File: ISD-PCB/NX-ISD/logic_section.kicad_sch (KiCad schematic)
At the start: 12 parts, among them J1 1-2328702-0, Q4 AO3400A, U1 ESP32-S3-WROOM-1, U14 ZDSD02GLGEAG

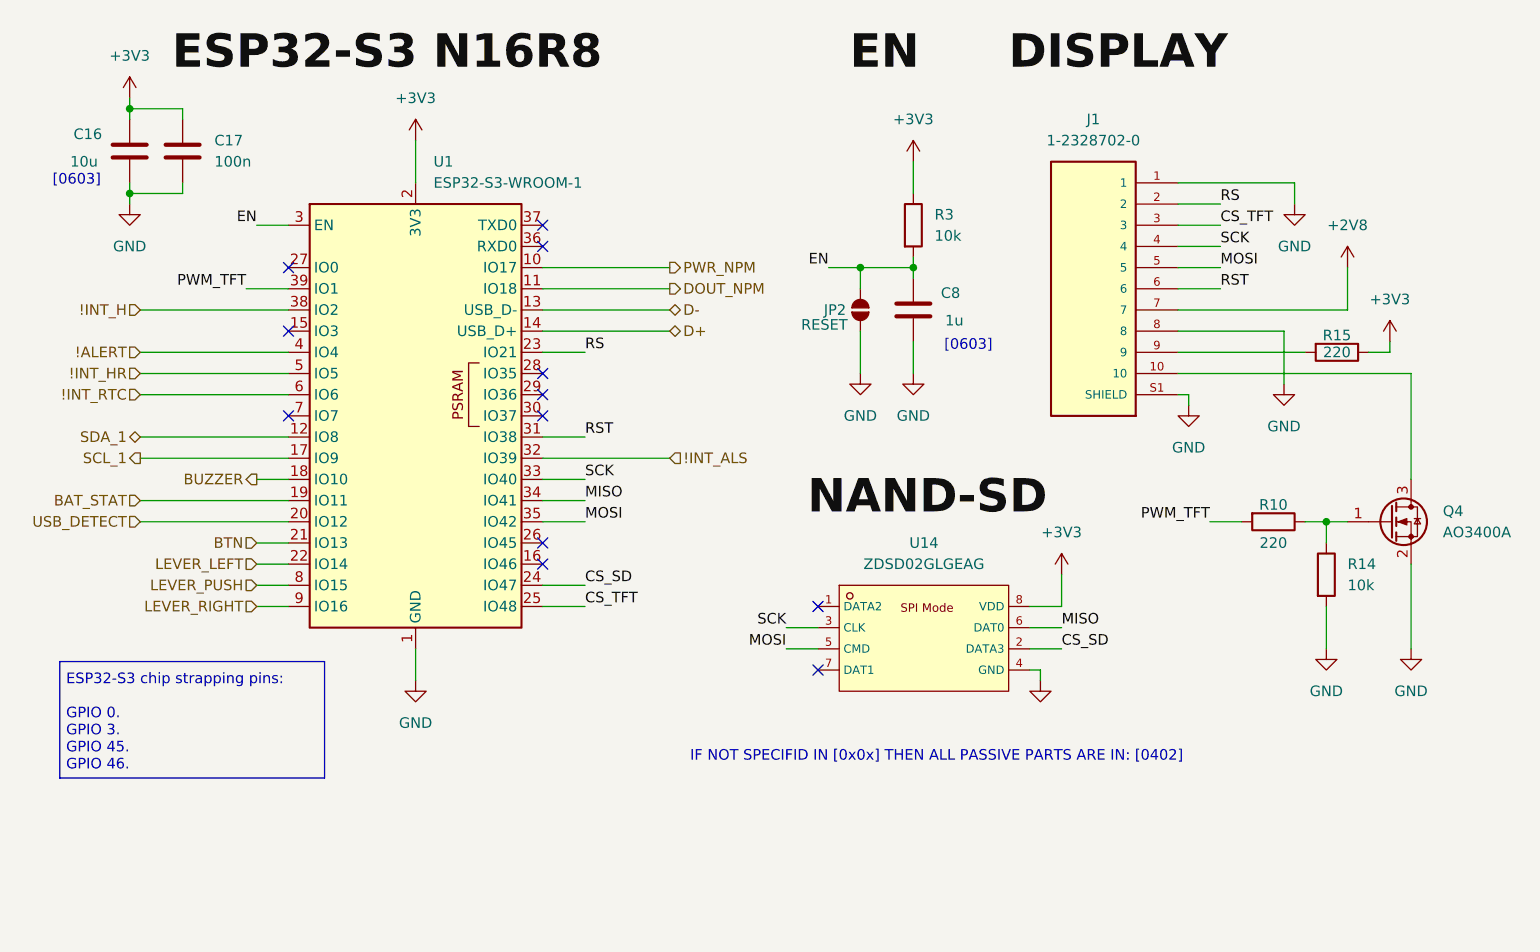
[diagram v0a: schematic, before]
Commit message: v1p1 rework in progress
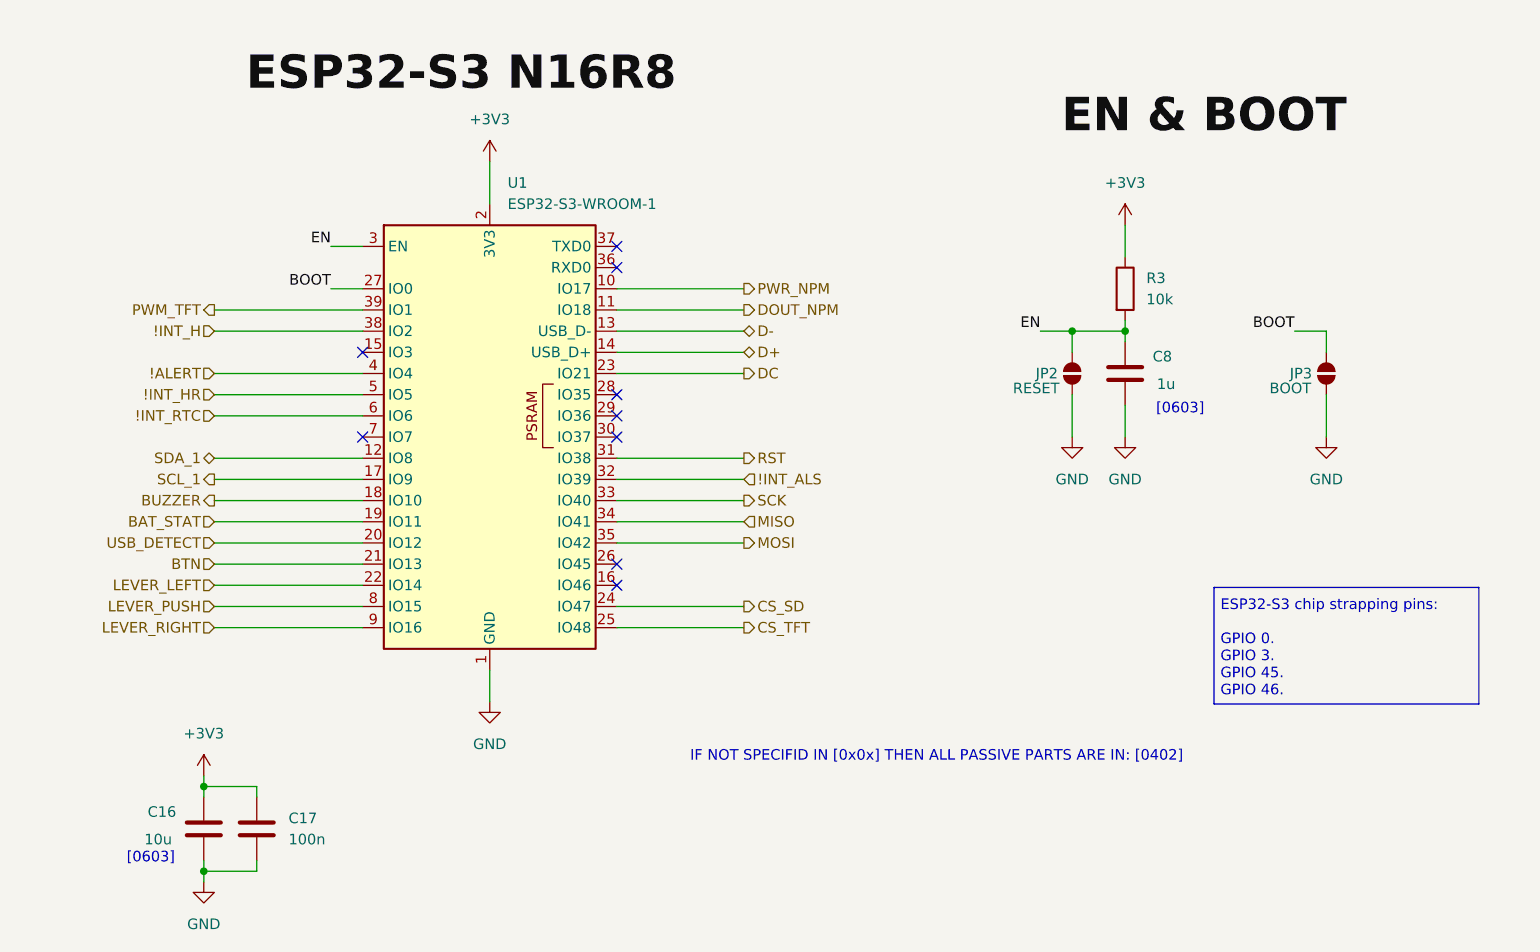
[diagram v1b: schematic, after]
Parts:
- removed J1: 1-2328702-0, Global Footprints:TE_1-2328702-0, symbol 1-2328702-0:1-2328702-0
- removed Q4: AO3400A, Package_TO_SOT_SMD:SOT-23, symbol Transistor_FET:AO3400A
- removed R10, R15: 220, Resistor_SMD:R_0402_1005Metric, symbol Device:R
- removed R14: 10k, Resistor_SMD:R_0402_1005Metric, symbol Device:R
- removed U14: ZDSD02GLGEAG, Global Footprints:LGA-8_L8.0-W6.0-P1.27-TL_ZDSD02GLGEAG, symbol ZDSD02GLGEAG:ZDSD02GLGEAG
- added JP3: BOOT, Jumper:SolderJumper-2_P1.3mm_Open_TrianglePad1.0x1.5mm, symbol Jumper:SolderJumper_2_Open
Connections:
- net GND: now also JP3.2 (B)
- net BOOT: now reaches U1.27 (IO0)
- net BOOT: now also JP3.1 (A)
- net RS renamed DC
- no-connect marks 12 -> 9
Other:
- moved on the sheet: C16, C17, C8, JP2, R3, U1
